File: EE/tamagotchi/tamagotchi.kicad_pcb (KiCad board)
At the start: 4 copper layers, 34.8 x 38.8 mm, 56 parts, among them J3 Conn_01x07, J7 TAG_CONNECT, P1 USB_C_Plug_USB2.0, Q1 Q_NMOS_GSD, Q2 Q_NMOS_GSD, Q3 Q_NMOS_GSD, Q4 Q_NMOS_GSD, Q5 Q_PMOS_GSD, Q7 Q_NMOS_GSD, SW2 TL1260BQRBLK, U2 STM32G031G8Ux

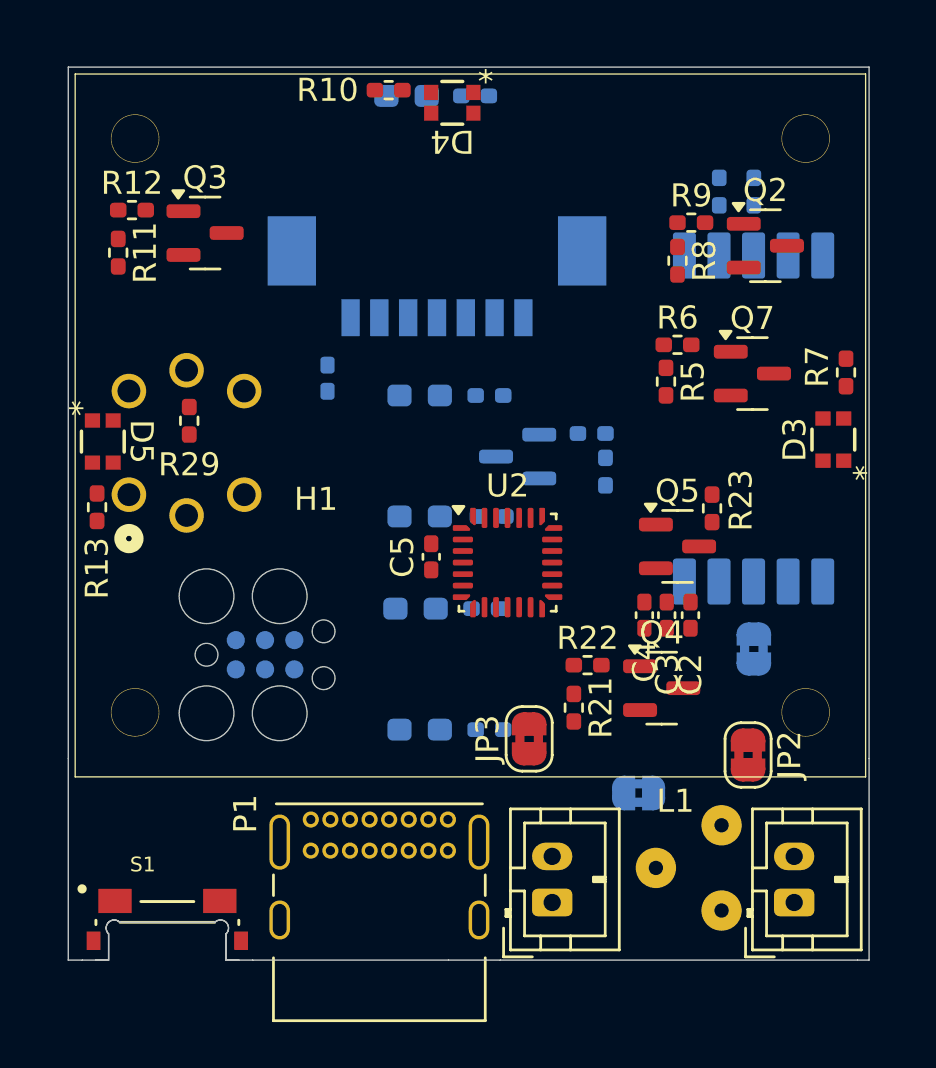
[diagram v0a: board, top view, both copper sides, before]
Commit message: Minor Placement update
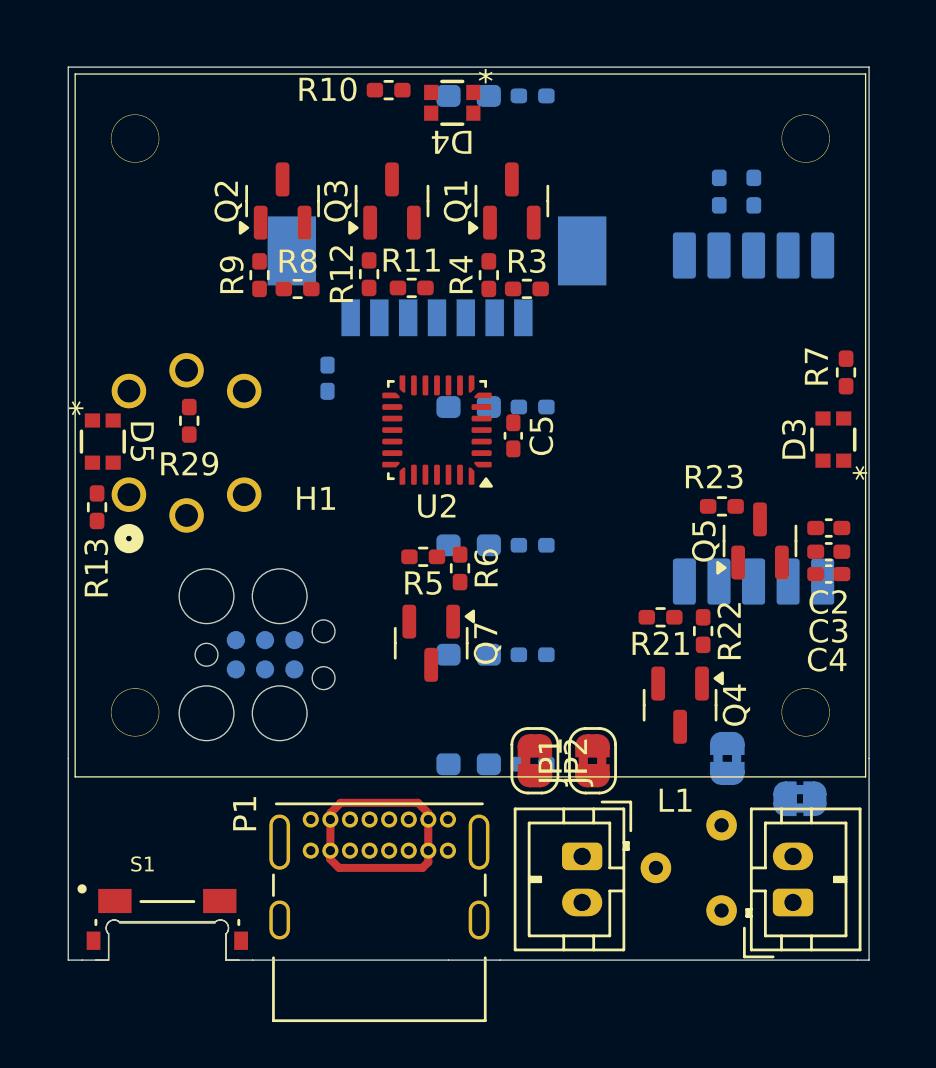
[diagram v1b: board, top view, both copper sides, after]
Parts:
- JP1, Q1, R3, R4: moved to F.Cu
- JP3: moved to B.Cu
- moved Q2 21.0 mm to (145.3, 76.8), turned to 90 degrees
- moved D1 19.7 mm to (153.4, 91.8)
- moved R2 19.7 mm to (156.2, 91.8)
- moved R9 18.9 mm to (144.3, 80.0), turned to 90 degrees
- moved Q7 18.2 mm to (151.8, 96.0), turned to -90 degrees
- moved R8 16.5 mm to (146.0, 80.6), turned to 0 degrees
- moved R6 13.5 mm to (153.0, 92.7), turned to -90 degrees
- moved D7 13.2 mm to (153.4, 72.2)
- moved R15 13.1 mm to (156.2, 72.2)
- moved R5 13.0 mm to (151.4, 92.2), turned to 180 degrees
- moved R11 12.8 mm to (150.9, 80.6), turned to 0 degrees
- moved Q1 11.1 mm to (155.2, 76.8), turned to 90 degrees
- moved R12 10.7 mm to (149.1, 80.0), turned to 90 degrees
- moved UT 10.4 mm to (167.4, 107.2)
- moved BATTERY 9.41 mm to (158.3, 105.2), turned to -90 degrees
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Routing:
- net VBUS: track 0.00 -> 13.3 mm
